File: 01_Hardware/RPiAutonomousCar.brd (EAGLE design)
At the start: 67.3 x 58.4 mm, 41 parts, among them IC1 7805TV, U1 TXB0108PWR, U2 SN74LVC1G04DCKR, U3 SN74LVC1G04DCKR, U4 MCP3004-I/ST

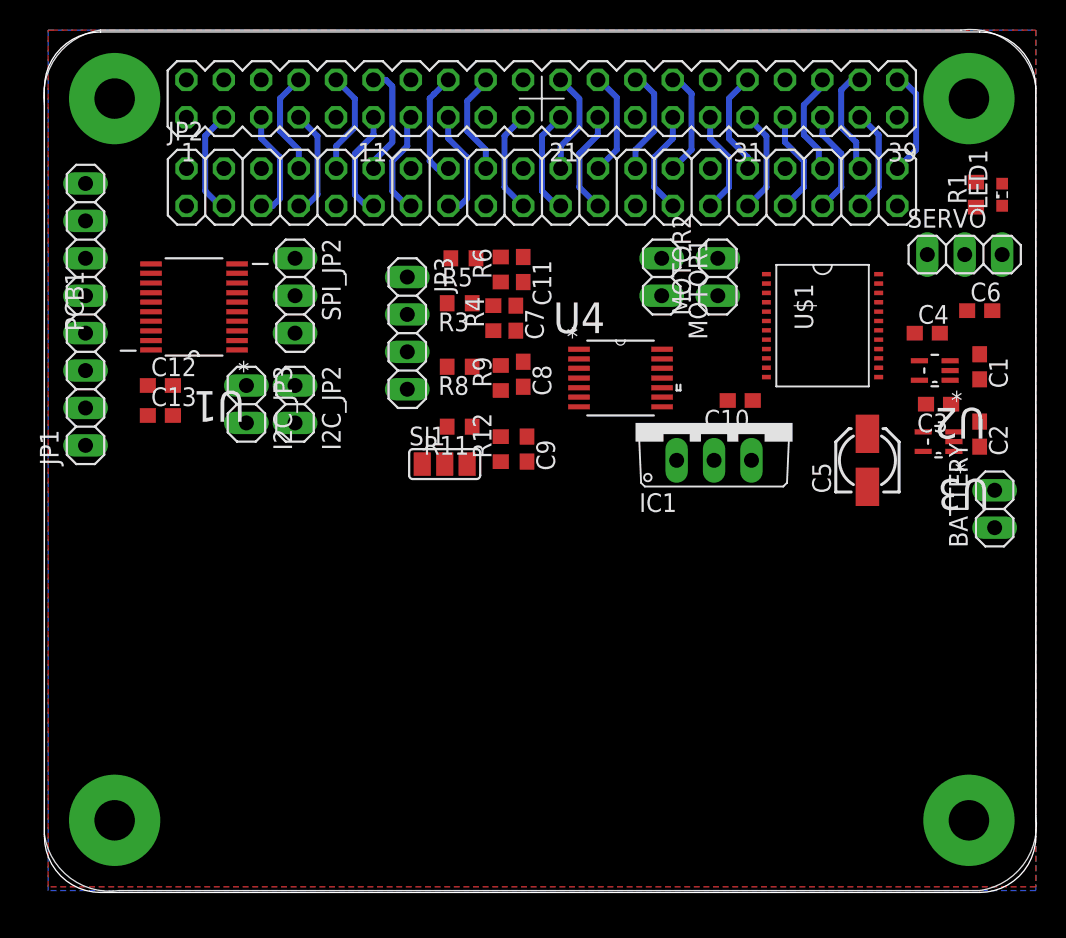
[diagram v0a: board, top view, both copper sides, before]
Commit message: routing ...
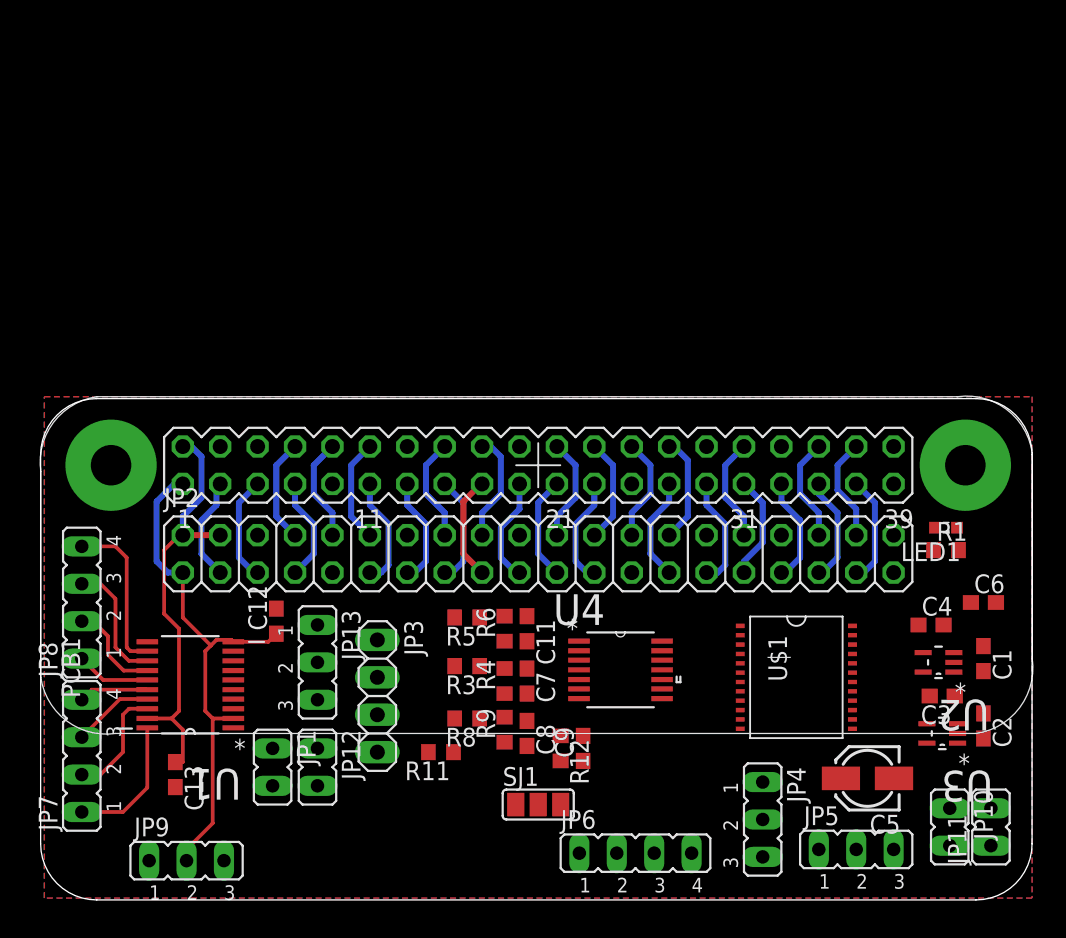
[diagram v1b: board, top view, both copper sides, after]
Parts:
- removed BATTERY, I2C_JP2, I2C_JP3, MOTOR1, MOTOR2: (no value), pinhead:1X02
- removed C10: 100n, rcl:C0603
- removed IC1: 7805TV, linear:TO220V
- removed SERVO, SPI_JP2: (no value), pinhead:1X03
- added JP10, JP11, JP12: (no value), jumper:JP1
- added JP13, JP4, JP5, JP9: (no value), jumper:JP2
- added JP6, JP7, JP8: (no value), jumper:JP4
- JP1: device pinhead:1X08 -> jumper:JP1
- PCB1: device RPiAutonomousCar:RASPBERRY_PI_BPLUS_DIM -> RPiAutonomousCar:RASPBERRY_PI_BPLUS_HEADER_ONLY
- moved PCB1 37.1 mm to (31.8, 20.1)
- moved JP1 33.3 mm to (15.7, 8.89), turned to 180 degrees
- moved U1 25.7 mm to (10.2, 14.5)
- moved JP2 24.9 mm to (33.8, 23.4)
- moved JP3 24.7 mm to (22.9, 13.7)
- moved C7 24.6 mm to (33.0, 14.7)
- moved R4 24.6 mm to (31.5, 14.7)
- moved R3 24.6 mm to (29.0, 15.7)
- moved C13 24.4 mm to (9.14, 8.38), turned to 270 degrees
- moved C8 24.4 mm to (33.0, 11.2)
- moved C11 24.4 mm to (33.0, 18.3)
- moved R5 24.4 mm to (29.0, 19.1)
- moved R6 24.4 mm to (31.5, 18.3)
- moved R1 24.2 mm to (61.5, 23.6), turned to 0 degrees
- moved SJ1 24.0 mm to (33.8, 6.35)
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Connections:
- removed net RPI14: U1.8
- removed net RPI17: JP2.17
- removed net SERVOPWM: SERVO.1
- net +3V3: now also JP2.17, JP6.4, JP9.2; no longer SERVO.2
- net +5V: now also JP5.2; no longer C10.1, IC1.3
- net +UB: now also JP4.2; no longer BATTERY.2, IC1.1
- net GND: now also JP4.1, JP4.3, JP5.1, JP5.3, JP6.1, JP9.3; no longer BATTERY.1, C10.2, IC1.2, SERVO.3
- net M1_OUT1: now also JP10.1; no longer MOTOR1.1
- net M1_OUT2: now also JP10.2; no longer MOTOR1.2
- net M2_OUT1: now also JP11.1; no longer MOTOR2.1
- net M2_OUT2: now also JP11.2; no longer MOTOR2.2
- net N$1: now also JP8.4; no longer JP1.8
- net N$16: now also JP9.1; no longer LED1.A
- net N$2: now also JP8.3; no longer JP1.7
- net N$3: now also JP8.2; no longer JP1.6
- net N$4: now also JP8.1; no longer JP1.5
- net N$5: now also JP7.4; no longer JP1.4
- net N$6: now also JP7.3; no longer JP1.3
- net N$7: now also JP7.2; no longer JP1.2
- net N$8: now also JP7.1; no longer JP1.1
- net RPI10: now also U1.9
- net RPI15: no longer U1.9
- net RPI19: now also JP13.3; no longer SPI_JP2.3
- net RPI21: now also JP13.2; no longer SPI_JP2.2
- net RPI23: now also JP13.1; no longer SPI_JP2.1
- net RPI3: now also JP1.2, JP12.2; no longer I2C_JP2.2, I2C_JP3.2
- net RPI40: now also LED1.A
- net RPI5: now also JP1.1, JP12.1; no longer I2C_JP2.1, I2C_JP3.1
- net RPI8: now also U1.8
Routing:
- net +3V3: track 0.00 -> 43.3 mm
- net +5V: track 0.00 -> 29.1 mm
- net N$1: track 0.00 -> 11.0 mm
- net N$8: track 0.00 -> 9.19 mm
- net N$2: track 0.00 -> 8.76 mm
- net N$7: track 0.00 -> 7.78 mm
- net RPI40: track 7.28 -> 0.00 mm
- net N$3: track 0.00 -> 6.58 mm
- net N$6: track 0.00 -> 5.52 mm
- net N$4: track 0.00 -> 5.04 mm
- net N$5: track 0.00 -> 4.73 mm
- net RPI12: track 7.57 -> 7.07 mm
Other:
- board size 67.3 x 58.4 mm -> 67.3 x 34 mm
